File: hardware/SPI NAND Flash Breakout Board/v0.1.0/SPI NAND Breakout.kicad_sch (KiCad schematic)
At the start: 7 parts, among them J1 Conn_01x08_Pin, U1 AS5F18G04SND-10LIN

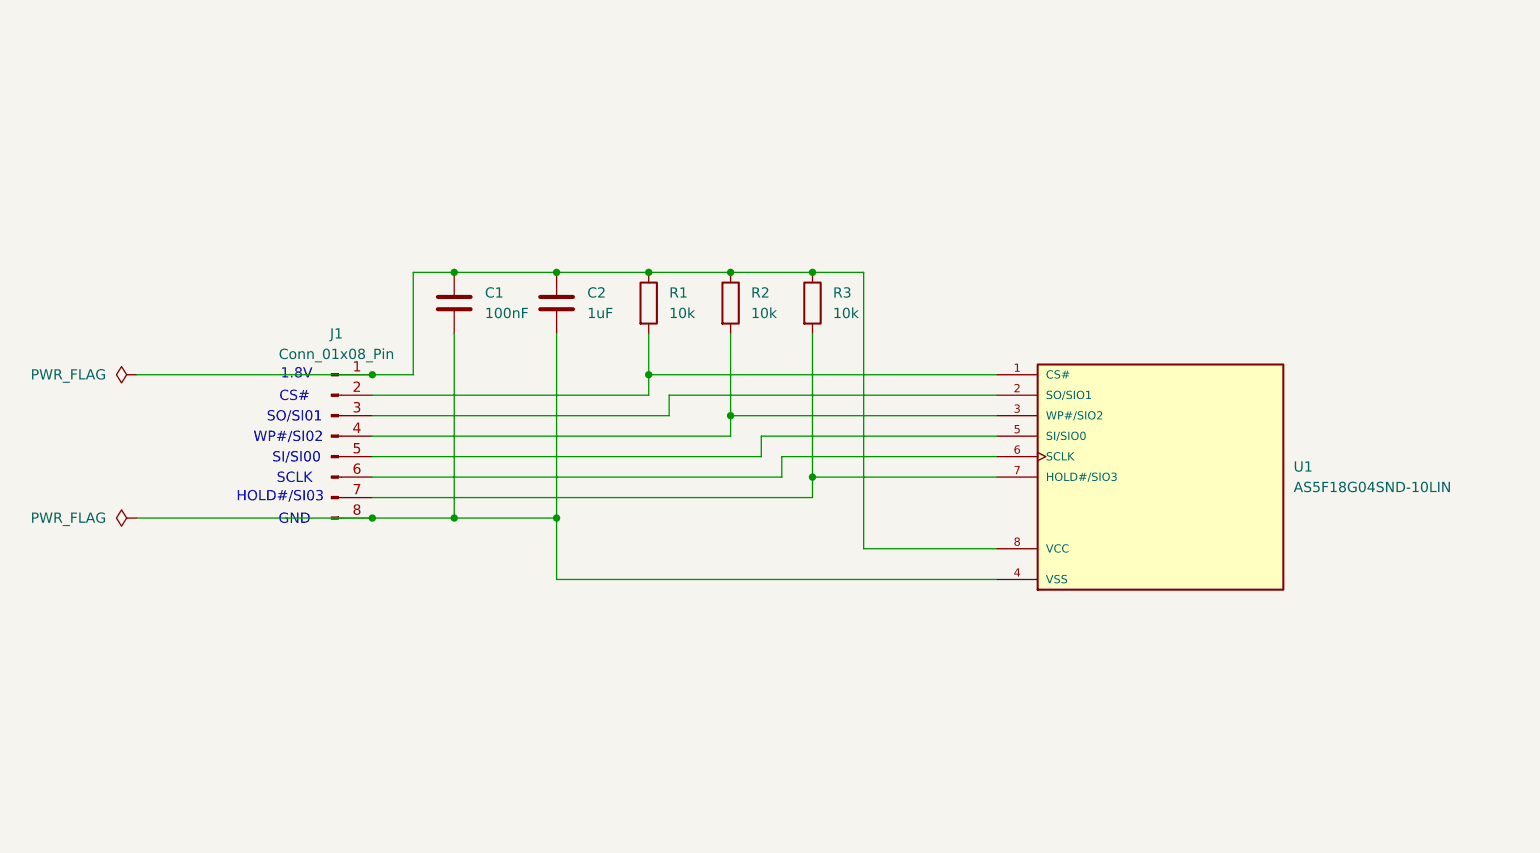
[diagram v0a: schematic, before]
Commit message: updated schematic
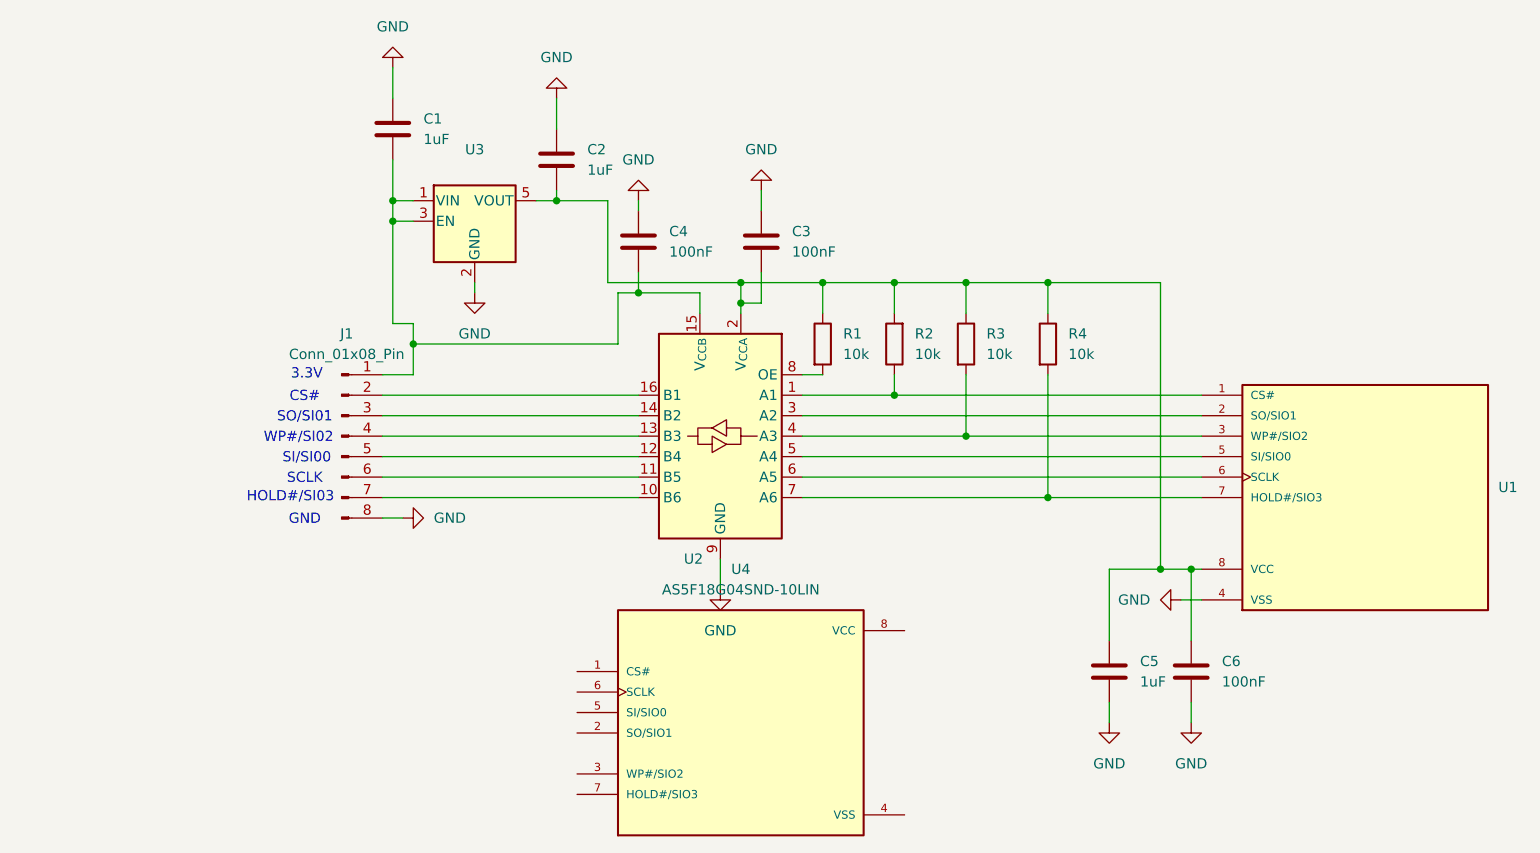
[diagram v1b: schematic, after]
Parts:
- added C3, C4, C6: 100nF, Capacitor_SMD:C_0805_2012Metric, symbol Device:C
- added C5: 1uF, Capacitor_SMD:C_0805_2012Metric, symbol Device:C
- added R4: 10k, Resistor_SMD:R_0805_2012Metric, symbol Device:R
- added U2: TXB0106PW, Package_SO:TSSOP-16_4.4x5mm_P0.65mm, symbol Logic_LevelTranslator:TXB0106PW
- added U3: AP2127K-1.8, Package_TO_SOT_SMD:SOT-23-5, symbol Regulator_Linear:AP2127K-1.8
- added U4: AS5F18G04SND-10LIN, AS5F18G04SND-10LIN:SON127P600X800X80-8N, symbol AS5F18G04SND-10LIN:AS5F18G04SND-10LIN
- C1: value 100nF -> 1uF; footprint Capacitor_SMD:C_0402_1005Metric -> Capacitor_SMD:C_0805_2012Metric
- C2: footprint Capacitor_SMD:C_0402_1005Metric -> Capacitor_SMD:C_0805_2012Metric
- R1, R2, R3: footprint Resistor_SMD:R_0402_1005Metric -> Resistor_SMD:R_0805_2012Metric
- U1: footprint AS5F18G04SND_10LIN:AS5F18G04SND-10LIN -> AS5F18G04SND-10LIN
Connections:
- net GND: now reaches J1.8 (Pin_8), U1.4 (VSS)
- net GND: now also C1.1, C2.1, C3.1, C4.1, C5.2, C6.2, U2.9 (GND), U3.2 (GND); no longer C1.2, C2.2
- net at J1.3 (Pin_3): now also U2.14 (B2); no longer U1.2 (SO/SIO1)
- net at J1.5 (Pin_5): now also U2.12 (B4); no longer U1.5 (SI/SIO0)
- net at J1.6 (Pin_6): now also U2.11 (B5); no longer U1.6 (SCLK)
- new net: C2.2, C3.2, C5.1, C6.1, R1.1, R2.2, R3.1, R4.1, U1.8 (VCC), U2.2 (V_{CCA}), U3.5 (VOUT)
- new net: R3.2, U1.3 (WP#/SIO2), U2.4 (A3)
- new net: R1.2, U2.8 (OE)
- new net: R2.1, U1.1 (CS#), U2.1 (A1)
- new net: J1.7 (Pin_7), U2.10 (B6)
- new net: J1.4 (Pin_4), U2.13 (B3)
- new net: C1.2, C4.2, J1.1 (Pin_1), U2.15 (V_{CCB}), U3.1 (VIN), U3.3 (EN)
- new net: J1.2 (Pin_2), U2.16 (B1)
- new net: U1.2 (SO/SIO1), U2.3 (A2)
- new net: U1.5 (SI/SIO0), U2.5 (A4)
- new net: U1.6 (SCLK), U2.6 (A5)
- new net: R4.2, U1.7 (HOLD#/SIO3), U2.7 (A6)
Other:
- note added: "3.3V"
- note removed: "1.8V"
- moved on the sheet: C1, C2, J1, R1, R2, R3, U1
